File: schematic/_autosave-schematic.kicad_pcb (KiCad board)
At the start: 4 copper layers, 44 x 112 mm, 6 parts, among them SW1 SW_Push

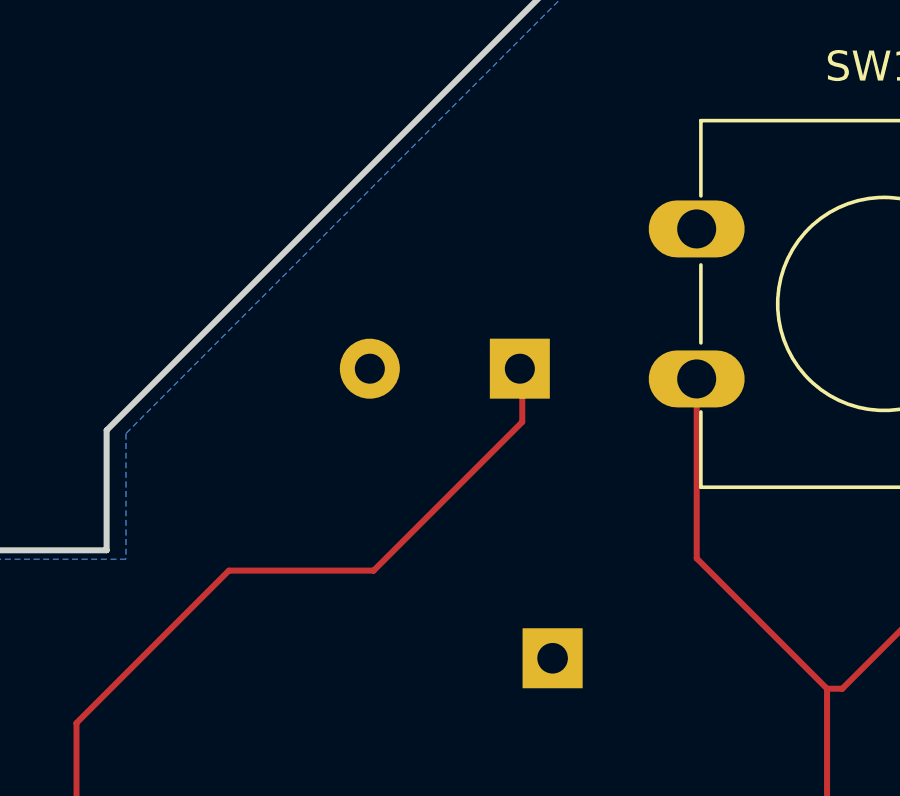
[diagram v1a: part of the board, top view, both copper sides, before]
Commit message: not touching fusion, this time for real
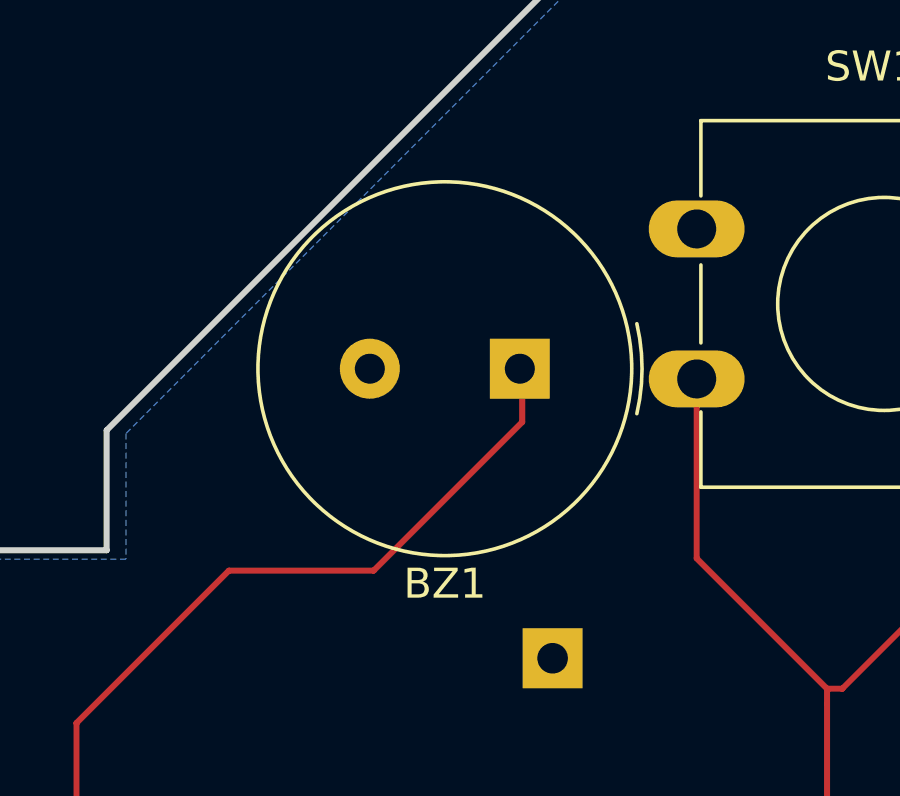
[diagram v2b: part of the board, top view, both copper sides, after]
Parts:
- BZ1: moved to F.Cu
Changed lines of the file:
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@@
 	)
 	(footprint "Buzzer_Beeper:Buzzer_TDK_PS1240P02BT_D12.2mm_H6.5mm"
-		(layer "B.Cu")
+		(layer "F.Cu")
 		(at 220.011 42.037 180)
 		(descr "Buzzer, D12.2mm height 6.5mm, https://product.tdk.com/info/en/catalog/datasheets/piezoelectronic_buzzer_ps_en.pdf")
 		(tags "buzzer")
 		(property "Reference" "BZ1"
-			(at 2.5 7.17 0)
-			(layer "B.SilkS")
+			(at 2.5 -7.17 0)
+			(layer "F.SilkS")
 			(effects
 				(font
@@
 					(thickness 0.15)
 				)
-				(justify mirror)
 			)
 		)
 		(property "Value" "Buzzer"
-			(at 2.5 -7.31 0)
-			(layer "B.Fab")
+			(at 2.5 7.31 0)
+			(layer "F.Fab")
 			(hide yes)
 			(effects
@@
 					(thickness 0.15)
 				)
-				(justify mirror)
 			)
 		)
 		(property "Datasheet" "~"
-			(at 0 0 0)
+			(at 0 0 180)
 			(unlocked yes)
-			(layer "B.Fab")
+			(layer "F.Fab")
 			(hide yes)
 			(effects
@@
 					(thickness 0.15)
 				)
-				(justify mirror)
 			)
 		)
 		(property "Description" "Buzzer, polarized"
-			(at 0 0 0)
+			(at 0 0 180)
 			(unlocked yes)
-			(layer "B.Fab")
+			(layer "F.Fab")
 			(hide yes)
 			(effects
@@
 					(thickness 0.15)
 				)
-				(justify mirror)
 			)
 		)
@@
 		(attr through_hole)
 		(fp_arc
-			(start -3.9 1.5)
+			(start -3.9 1.499999)
 			(mid -4.073431 0)
-			(end -3.9 -1.499999)
+			(end -3.9 -1.5)
 			(stroke
 				(width 0.12)
 				(type solid)
 			)
-			(layer "B.SilkS")
+			(layer "F.SilkS")
 		)
 		(fp_circle
@@
 			)
 			(fill no)
-			(layer "B.SilkS")
+			(layer "F.SilkS")
 		)
 		(fp_circle
@@
 			)
 			(fill no)
-			(layer "B.CrtYd")
+			(layer "F.CrtYd")
 		)
 		(fp_line
-			(start -1.3 1)
-			(end -1.3 -1)
+			(start -1.3 -1)
+			(end -1.3 1)
 			(stroke
 				(width 0.1)
 				(type solid)
 			)
-			(layer "B.Fab")
+			(layer "F.Fab")
 		)
 		(fp_circle
@@
 			)
 			(fill no)
-			(layer "B.Fab")
+			(layer "F.Fab")
 		)
 		(fp_circle
@@
 			)
 			(fill no)
-			(layer "B.Fab")
+			(layer "F.Fab")
 		)
 		(pad "1" thru_hole rect
